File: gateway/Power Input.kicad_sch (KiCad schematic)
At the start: 21 parts, among them IC701 TPS2121RUXT, IC702 INA219AxD, Q701 BSS123, X701 DC In

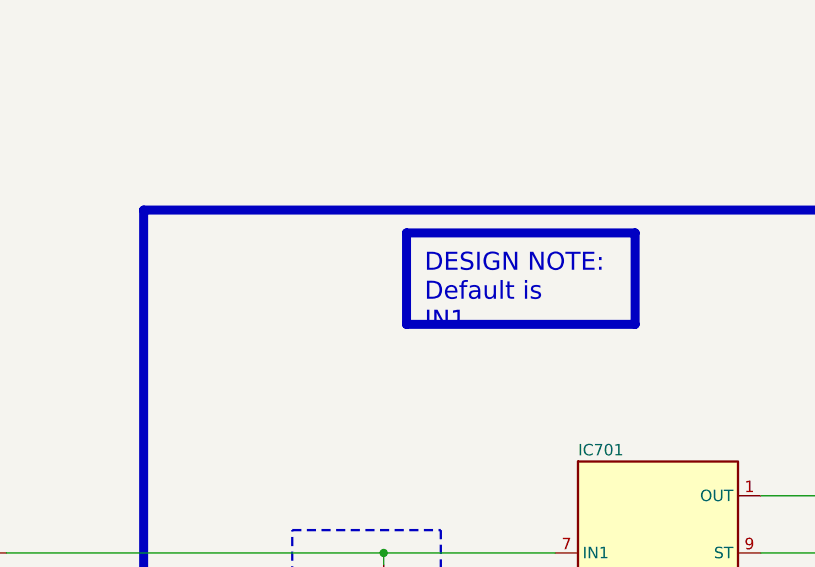
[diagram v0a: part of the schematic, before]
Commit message: Working on layout
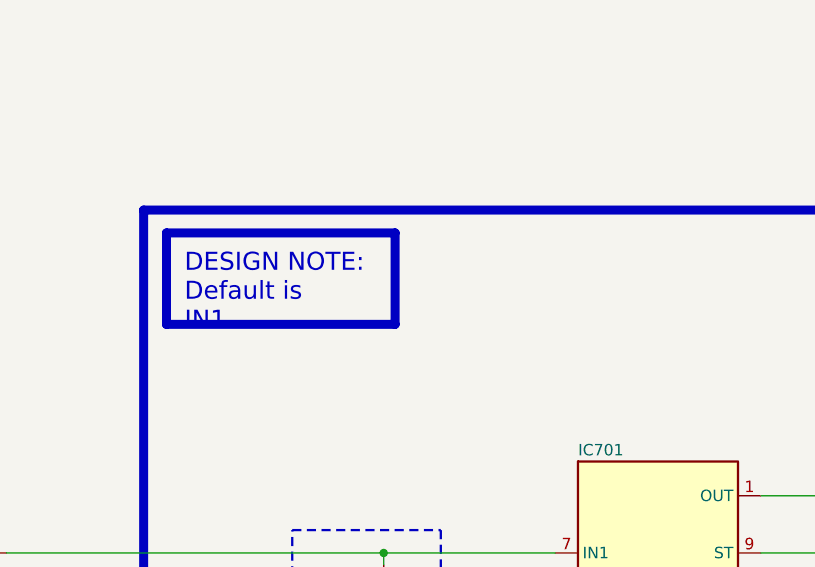
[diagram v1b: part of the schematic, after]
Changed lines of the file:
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@@
 	(text_box "DESIGN NOTE:\nDefault is IN1."
 		(exclude_from_sim no)
-		(at 92.71 138.43 0)
+		(at 66.04 138.43 0)
 		(size 25.4 10.16)
 		(margins 2 2 2 2)
